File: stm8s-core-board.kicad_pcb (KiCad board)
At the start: 2 copper layers, 23.9 x 23.9 mm, 21 parts, among them IC1 STM8S003F3P, P1 CONN_01X06, P2 USB_OTG, P3 CONN_01X09, P4 CONN_01X09, P5 CONN_01X02, SW1 SW_PUSH, U1 AS1117-5.0, Y1 16MHz

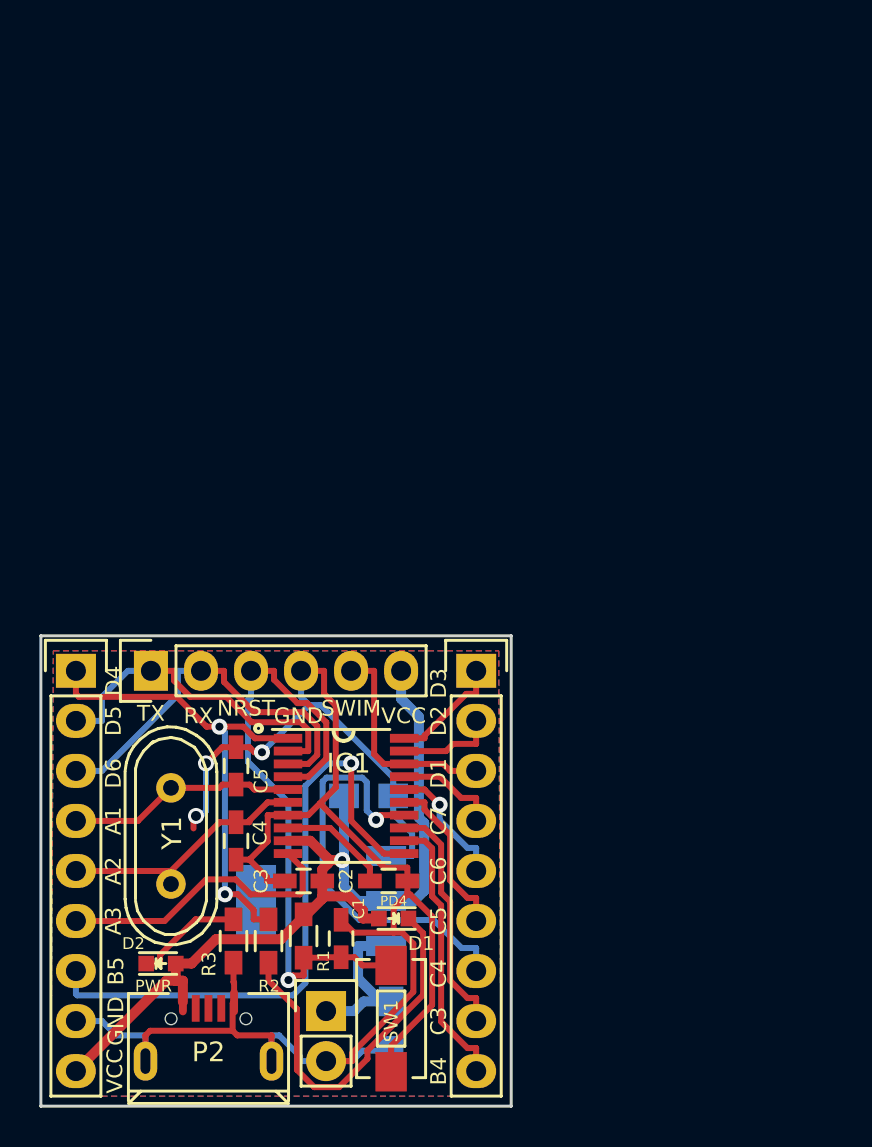
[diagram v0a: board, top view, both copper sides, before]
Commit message: forgot commit for long time. don't know what changed
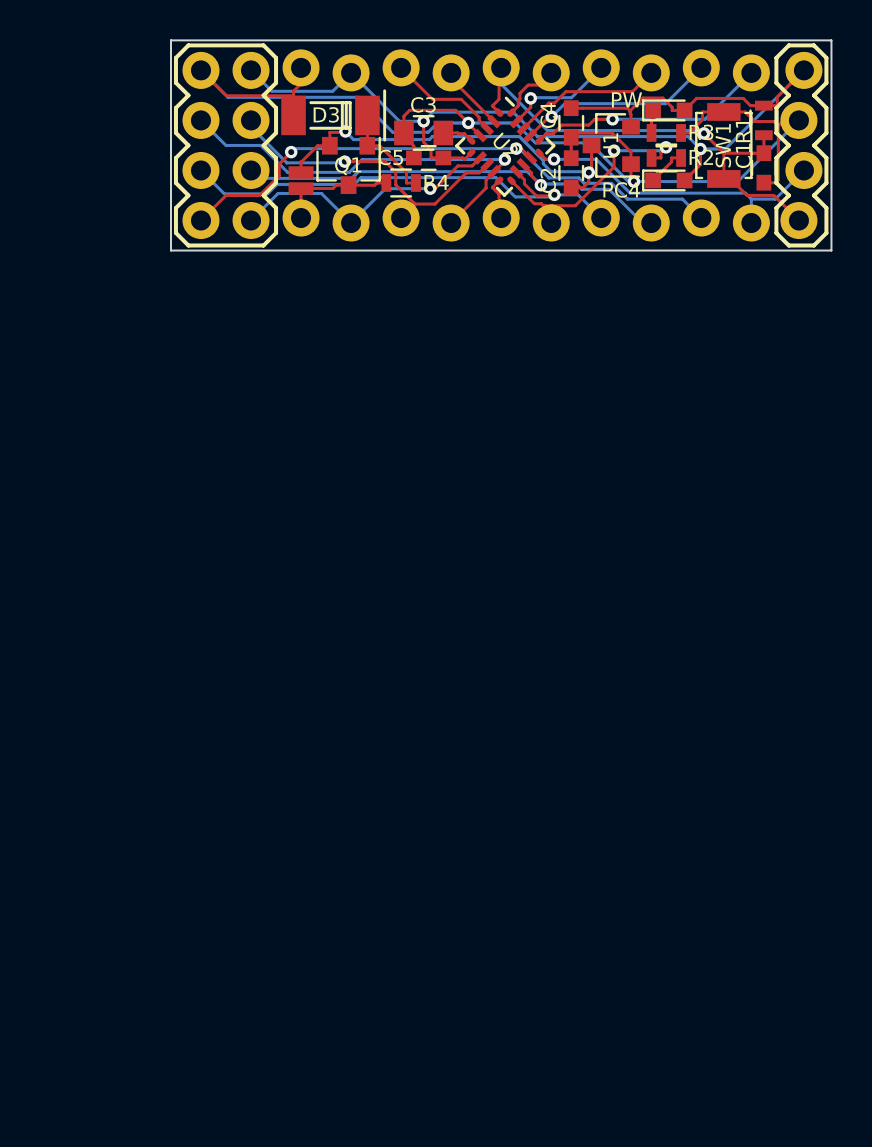
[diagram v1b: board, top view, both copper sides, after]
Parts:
- removed C6, C7: 10uF, Capacitors_SMD:C_0805_HandSoldering
- removed IC1: STM8S003F3P, Housings_SSOP:TSSOP-20_4.4x6.5mm_Pitch0.65mm
- removed P1: CONN_01X06, Pin_Headers:Pin_Header_Straight_1x06
- removed P2: USB_OTG, USB_Micro-B_MK5P
- removed P3, P4: CONN_01X09, Pin_Headers:Pin_Header_Straight_1x09
- removed P5: CONN_01X02, Pin_Headers:Pin_Header_Straight_1x02
- removed Y1: 16MHz, Crystals:Crystal_HC49-U_Vertical
- added D3: 5.6V, MyOwn:SOD-80, F.Cu at (159.0, 93.7)
- added J1: CONN_01X04, SparkFun-Connectors:1X04_LOCK, F.Cu at (182.9, 99.1)
- added J2: CONN_02X04, SparkFun-Connectors:2X4, F.Cu at (153.7, 95.2)
- added J3: CONN_01X10, SparkFun-Connectors:1X10_LOCK_NS, F.Cu at (157.5, 99.1)
- added J4: CONN_01X10, SparkFun-Connectors:1X10_LOCK_NS, F.Cu at (157.5, 91.4)
- added JP2: 12V-30V input, SparkFun-Jumpers:SMT-JUMPER_2_NO_NO-SILK, F.Cu at (157.5, 97.0)
- added Q1: BC817-40, TO_SOT_Packages_SMD:SOT-23, F.Cu at (159.9, 96.3)
- added R4: 1K, Resistors_SMD:R_0603, F.Cu at (162.6, 97.2)
- added U2: STM8S003F3U, MyOwn:UQFN-16_3x3mm_Pitch0.5mm, F.Cu at (167.8, 95.3)
- C1: footprint Capacitors_SMD:C_0603_HandSoldering -> Capacitors_SMD:C_0603
- C2: value 1.0uF -> 1uF; footprint Capacitors_SMD:C_0603_HandSoldering -> Capacitors_SMD:C_0603
- C3: value 0.1uF -> 1.0uF; footprint Capacitors_SMD:C_0603_HandSoldering -> Capacitors_SMD:C_0805
- C4: value 22pF -> 1uF; footprint Capacitors_SMD:C_0603_HandSoldering -> Capacitors_SMD:C_0603
- C5: value 22pF -> 0.1uF; footprint Capacitors_SMD:C_0603_HandSoldering -> Capacitors_SMD:C_0603
- D1, D2: footprint LEDs:LED-0603 -> LEDs:LED_0603
- R1, R2, R3: footprint Resistors_SMD:R_0603_HandSoldering -> Resistors_SMD:R_0603
- SW1: footprint Buttons_Switches_SMD:SW_SPST_EVQPE1 -> Buttons_Switches_SMD:SW_SPST_B3U-1000P
- U1: value AS1117-5.0 -> XC6206; footprint TO_SOT_Packages_SMD:SOT-223 -> TO_SOT_Packages_SMD:SOT-23; moved to F.Cu
- moved D2 50.4 mm to (176.1, 93.5)
- moved R1 47.5 mm to (181.0, 94.0)
- moved SW1 47.4 mm to (178.9, 95.2), turned to 90 degrees
- moved R3 46.5 mm to (176.0, 94.6), turned to 0 degrees
- moved C1 44.6 mm to (181.0, 96.4), turned to 270 degrees
- moved R2 44.6 mm to (176.0, 95.9), turned to 180 degrees
- moved U1 41.1 mm to (173.2, 95.2), turned to 180 degrees
- moved C4 40.2 mm to (171.2, 94.1)
- moved D1 40.0 mm to (176.1, 97.0), turned to 0 degrees
- moved C3 38.5 mm to (163.7, 94.6), turned to 180 degrees
- moved C2 37.1 mm to (171.2, 96.6), turned to 90 degrees
- moved C5 32.4 mm to (164.0, 95.9), turned to 0 degrees
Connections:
- C3 pad 1: GND -> Net-(C3-Pad1)
- C3 pad 2: VCC -> GND
- C4 pad 1: PA2/OSC_OUT -> +3V3
- C5 pad 1: PA1/OSC_IN -> GND
- C5 pad 2: GND -> +3V3
- D1 pad 2: VCC -> +3V3
- D2 pad 2: VCC -> +3V3
- R1 pad 1: VCC -> +3V3
- R2 pad 2: PD4 -> PC4
- U1 pad 2: VCC -> +3V3
- U1 pad 3: +12V -> Net-(C2-Pad1)
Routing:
- net +3V3: track 0.00 -> 53.4 mm, vias 0 -> 2
- net VCC: track 48.0 -> 5.94 mm, vias 1 -> 0
- net GND: track 99.6 -> 65.8 mm, vias 3 -> 2
- net PC7: track 5.27 -> 29.6 mm, vias 0 -> 2
- net Net-(D1-Pad1): track 19.2 -> 2.01 mm
- net PD4: track 24.5 -> 7.66 mm, vias 2 -> 0
- net PC6: track 6.51 -> 23.2 mm
- net PD6/RX: track 19.7 -> 3.17 mm
- net PC5: track 8.40 -> 24.7 mm, vias 0 -> 1
- net PB5: track 32.2 -> 16.2 mm
- net Net-(C2-Pad1): track 5.67 -> 20.2 mm, vias 0 -> 2
- net PD5/TX: track 17.2 -> 5.70 mm, vias 0 -> 1
- net PC3: track 12.2 -> 2.21 mm
- net PC4: track 21.5 -> 12.1 mm, vias 1 -> 2
- net PA1/OSC_IN: track 11.6 -> 3.38 mm
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- removed copper zone on B.Cu, net GND
- removed copper zone on F.Cu, net GND
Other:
- board size 23.9 x 23.9 mm -> 33.5 x 10.7 mm
- net class +12V removed
- net class Default: trace_width 0.3048 -> 0.1524; via_dia 0.8128 -> 0.635; via_drill 0.508 -> 0.3
- net class VCC removed
- rule pad_to_mask_clearance: 0.2 -> 0
- rule via_min_drill: 0.3048 -> 0.3
- rule via_min_size: 0.6096 -> 0.635
- board text added: "3V3"
- board text added: "G"
- board text added: "PC4"
- board text added: "PW"
- board text added: "RS"
- board text added: "RST"
- board text added: "S"
- board text added: "SW"
- board text removed: "+12V INPUT"
- board text removed: "C6"
- board text removed: "D1"
- board text removed: "NRST"
- board text removed: "PD4"
- board text removed: "PWR"
- board text removed: "RX"
- board text removed: "Rev1.0 Dec-2015 Designed by HW Wong"
- board text removed: "SWIM"
- board text removed: "TX"
